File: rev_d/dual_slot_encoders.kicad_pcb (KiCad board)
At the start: 2 copper layers, 50 x 25 mm, 16 parts, among them U1 GP1S094HCZ0F, U2 GP1S094HCZ0F, U3 GPS1S97HCZ0F, U4 GPS1S97HCZ0F

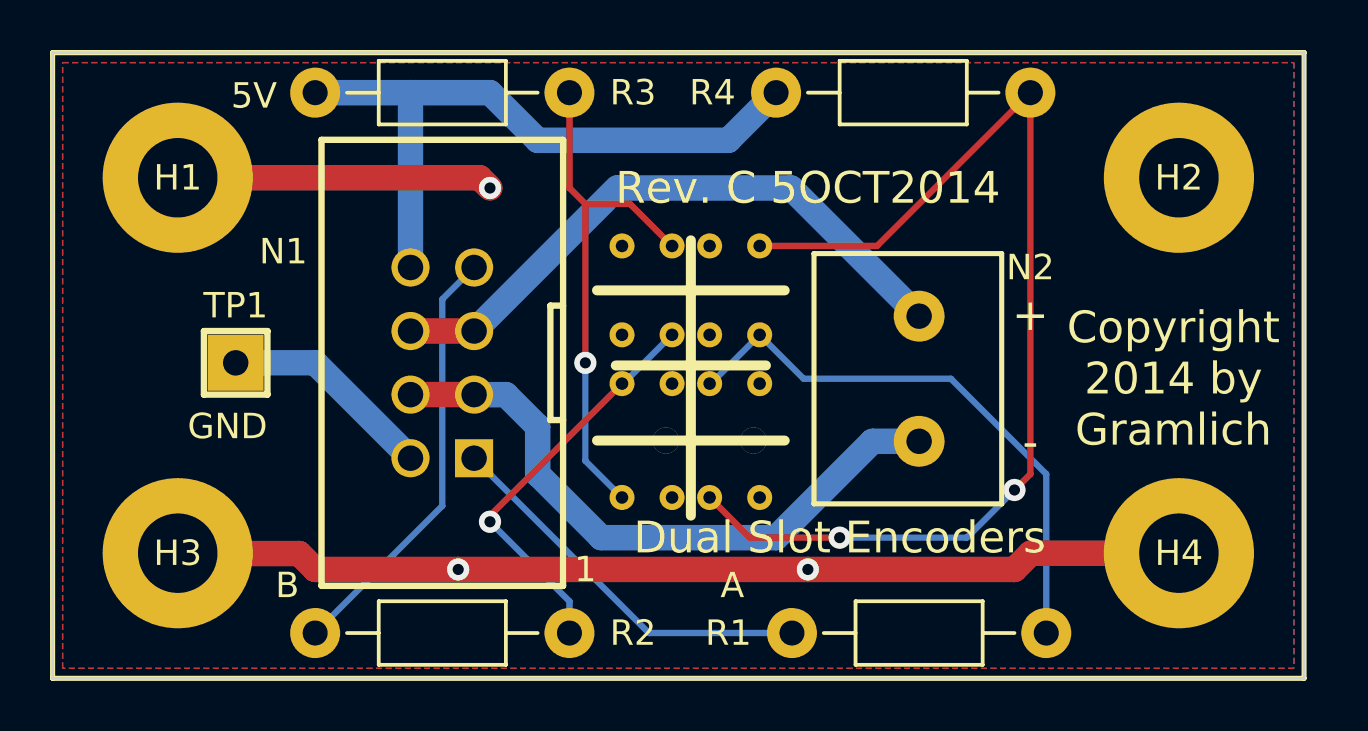
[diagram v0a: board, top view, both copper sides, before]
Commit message: Rev. D is pretty much ready.
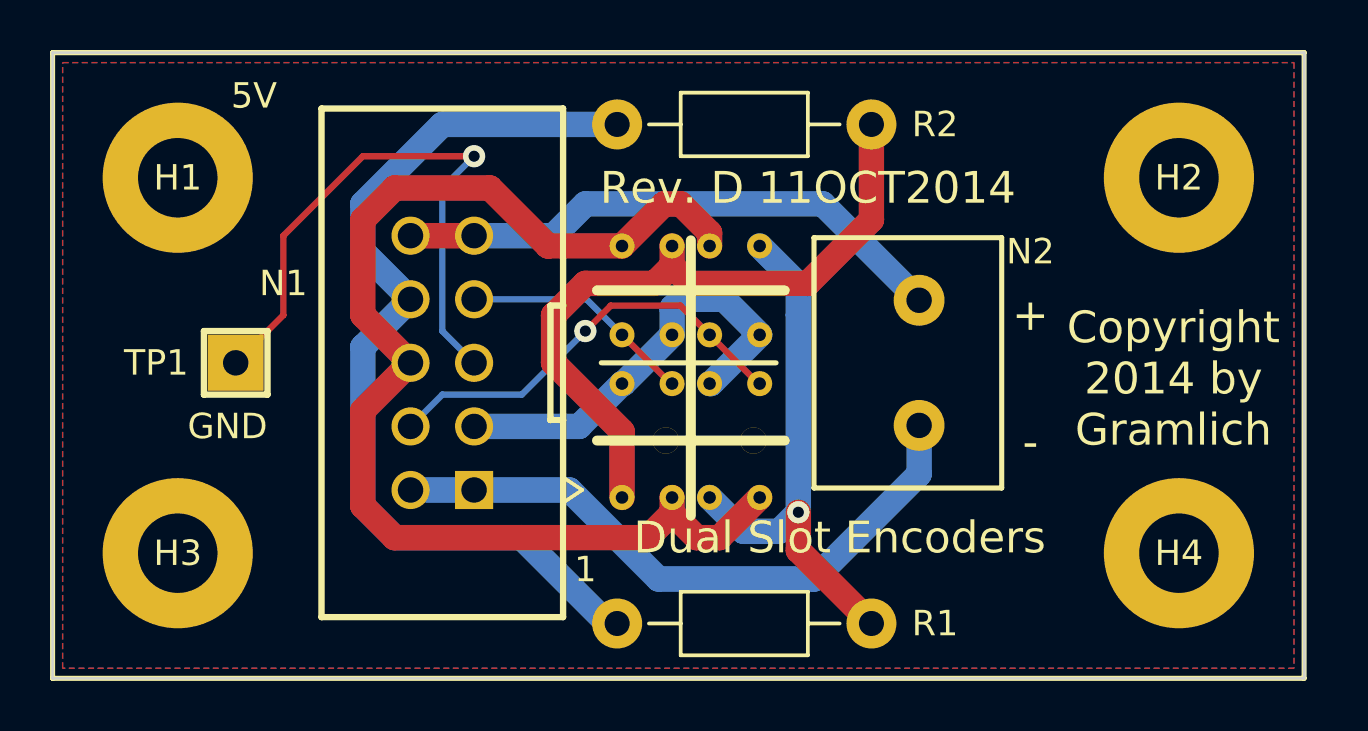
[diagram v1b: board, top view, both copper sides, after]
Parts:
- removed R3, R4: 470, dual_slot_encoders:Resistor_Horizontal_400
- N1: value MOTOR_ENCODER_CONN -> MOTOR_ENCODER_CONN_2X5; footprint dual_slot_encoders:Pin_Header_Straight_2x04_Shrouded -> dual_slot_encoders:Pin_Header_Straight_2x05_Shrouded
- R1, R2: value 10K -> 100
- moved R2 23.6 mm to (127.6, 102.9)
- moved R1 7.00 mm to (127.6, 122.8)
- moved N2 0.64 mm to (134.6, 112.4)
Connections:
- H1 pad 1: /GND -> /LGND
- H2 pad 1: /GND -> /LGND
- H3 pad 1: /GND -> /LGND
- H4 pad 1: /GND -> /LGND
- N1 pad 1: /A -> /MOTOR+
- N1 pad 2: /GND -> /MOTOR+
- N1 pad 3: /MOTOR- -> /LPWR
- N1 pad 4: /MOTOR- -> /A
- N1 pad 5: /MOTOR+ -> /LGND
- N1 pad 6: /MOTOR+ -> /LED_EN
- N1 pad 8: /5V -> /BPWR
- N2 pad 1: /MOTOR- -> /MOTOR+
- N2 pad 2: /MOTOR+ -> /MOTOR-
- R1 pad 2: /A -> /BPWR
- R2 pad 2: /B -> /BPWR
- TP1 pad 1: /GND -> /LGND
- U1 pad 1: Net-(R3-Pad1) -> Net-(R2-Pad1)
- U1 pad 2: Net-(R2-Pad1) -> /LPWR
- U1 pad 3: /GND -> /B
- U1 pad 4: /GND -> /LED_EN
- U2 pad 1: Net-(R4-Pad1) -> Net-(R1-Pad1)
- U2 pad 2: Net-(R1-Pad1) -> /LPWR
- U2 pad 3: /GND -> /A
- U2 pad 4: /GND -> /LED_EN
- U3 pad 1: Net-(R3-Pad1) -> Net-(R2-Pad1)
- U3 pad 2: Net-(R2-Pad1) -> /LPWR
- U3 pad 3: /GND -> /B
- U3 pad 4: /GND -> /LED_EN
- U4 pad 1: Net-(R4-Pad1) -> Net-(R1-Pad1)
- U4 pad 2: Net-(R1-Pad1) -> /LPWR
- U4 pad 3: /GND -> /A
- U4 pad 4: /GND -> /LED_EN
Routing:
- net /GND: track 61.7 -> 0.00 mm, vias 3 -> 0
- net /LED_EN: track 0.00 -> 48.5 mm
- net Net-(R4-Pad1): track 43.1 -> 0.00 mm, vias 2 -> 0
- net /BPWR: track 0.00 -> 37.2 mm
- net /5V: track 27.0 -> 0.00 mm
- net /LGND: track 0.00 -> 24.1 mm, vias 0 -> 1
- net Net-(R3-Pad1): track 21.2 -> 0.00 mm, vias 1 -> 0
- net /LPWR: track 0.00 -> 18.0 mm
- net Net-(R2-Pad1): track 16.3 -> 27.9 mm, vias 1 -> 0
- net /B: track 17.2 -> 9.31 mm
- net /MOTOR-: track 25.4 -> 22.4 mm
- net /A: track 15.6 -> 17.2 mm, vias 0 -> 1
- net Net-(R1-Pad1): track 22.9 -> 21.4 mm, vias 0 -> 1
- net /MOTOR+: track 24.8 -> 25.5 mm
- added copper zone on B.Cu, net /LGND
- added copper zone on F.Cu, net /LGND
- removed copper zone on B.Cu, net /GND
- removed copper zone on F.Cu, net /GND
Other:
- board text added: "Rev. D 11OCT2014"
- board text removed: "A"
- board text removed: "B"
- board text removed: "Rev. C 5OCT2014"
